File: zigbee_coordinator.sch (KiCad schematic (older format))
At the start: 51 parts, among them J1 USB_C_Receptacle_USB2.0, J2 SWD_POGO_PADS, J3 UART_POGO_PADS, J4 SWD_POGO, J5 SWD_CASTELLATED, J6 UART_CASTELLATED, J7 UART_POGO, Q1 Q_PMOS_GSD, Q2 2N7002, U1 93LCxxBxxOT, U2 MCP1603-OS, U3 FT232H, U4 74LVC126, Y1 12MHz

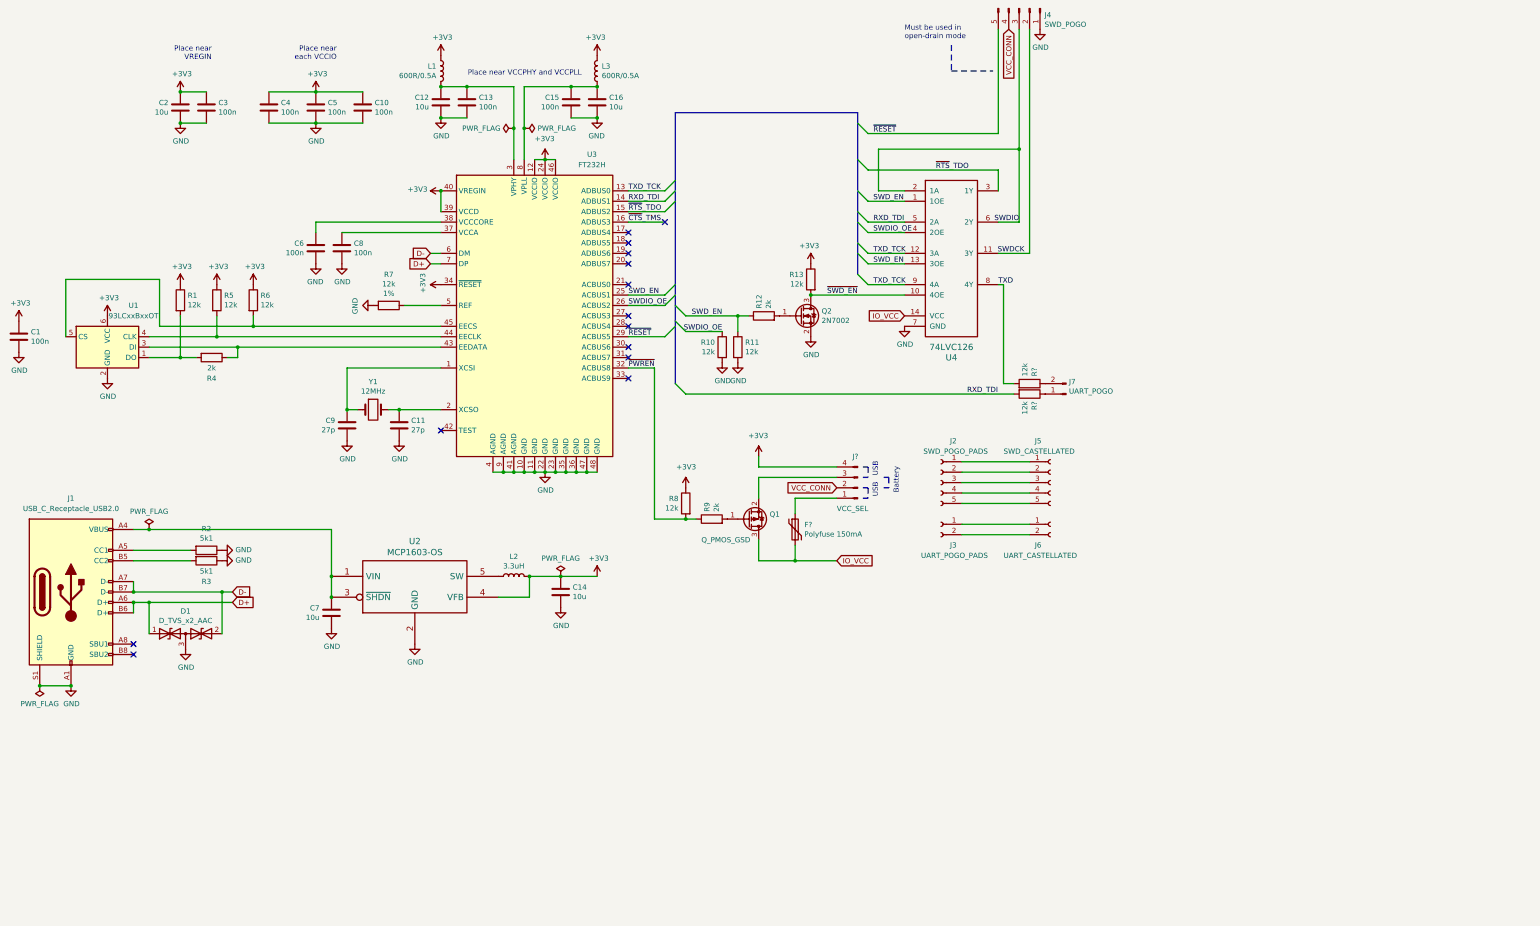
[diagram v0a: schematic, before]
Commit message: First alpha release
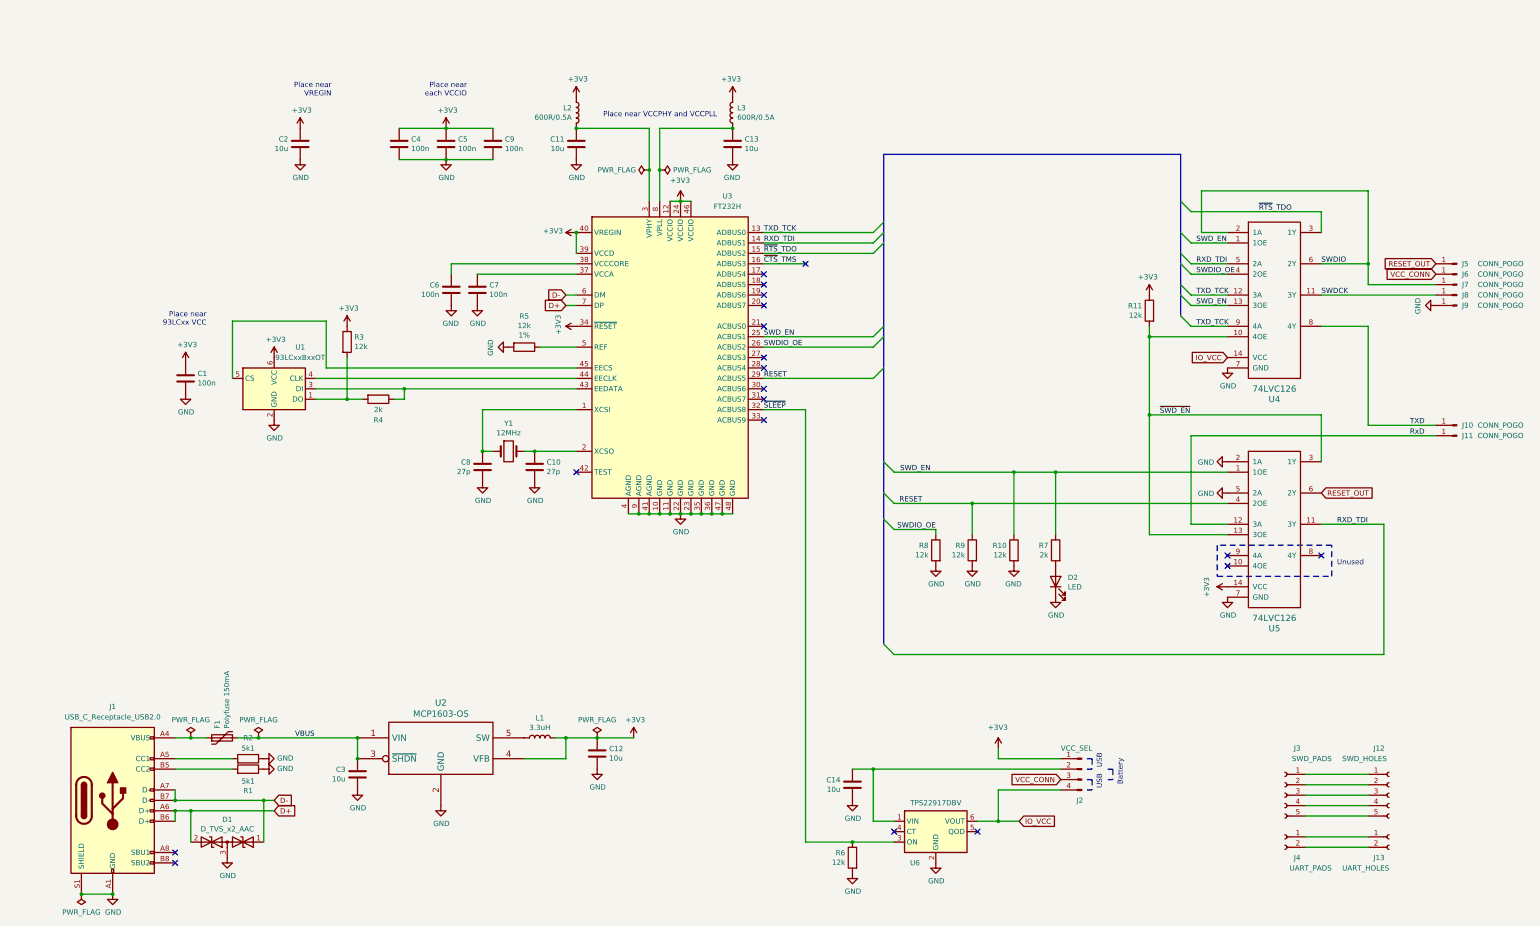
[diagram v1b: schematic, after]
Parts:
- removed C13, C15, C3: 100n, Capacitor_SMD:C_0805_2012Metric, symbol Device:C
- removed J2: SWD_POGO_PADS, symbol Connector:Conn_01x05_Female
- removed J3: UART_POGO_PADS, symbol Connector:Conn_01x02_Female
- removed J4: SWD_POGO, symbol Connector:Conn_01x05_Male
- removed J7: UART_POGO, symbol Connector:Conn_01x02_Male
- removed Q1: Q_PMOS_GSD, Inductor_SMD:L_0805_2012Metric, symbol Device:Q_PMOS_GSD
- removed Q2: 2N7002, Package_TO_SOT_SMD:SOT-23, symbol Transistor_FET:2N7002
- removed R12, R9: 2k, Resistor_SMD:R_0805_2012Metric, symbol Device:R
- removed R5, R6, R? (x2): 12k, Resistor_SMD:R_0805_2012Metric, symbol Device:R
- added C14: 10u, Capacitor_SMD:C_0805_2012Metric, symbol Device:C
- added D2: LED, LED_SMD:LED_0805_2012Metric, symbol Device:LED
- added J10, J11, J5, J6, J7, J8, J9: CONN_POGO, pogopin:pogopin, symbol Connector:Conn_01x01_Male
- added J3: SWD_PADS, pogopin:SWD_pads, symbol Connector:Conn_01x05_Female
- added J4: UART_PADS, pogopin:UART_pads, symbol Connector:Conn_01x02_Female
- added R10: 12k, Resistor_SMD:R_0805_2012Metric, symbol Device:R
- added R7: 2k, Resistor_SMD:R_0805_2012Metric, symbol Device:R
- added U5: 74LVC126, Package_SO:TSSOP-14_4.4x5mm_P0.65mm, symbol 74hc126:74HC126
- added U6: TPS22917DBV, Package_TO_SOT_SMD:SOT-23-6, symbol Power_Management:TPS22917DBV
- F1: renamed from F?; footprint (none) -> Fuse:Fuse_0805_2012Metric
- J12: renamed from J5; value SWD_CASTELLATED -> SWD_HOLES; footprint (none) -> pogopin:SWD_holes
- J13: renamed from J6; value UART_CASTELLATED -> UART_HOLES; footprint (none) -> pogopin:UART_holes
- J2: renamed from J?; footprint (none) -> Connector_PinHeader_1.27mm:PinHeader_1x04_P1.27mm_Horizontal
- Y1: footprint Crystal:Crystal_SMD_HC49-SD -> Crystal:Crystal_SMD_0603-2Pin_6.0x3.5mm
- renumbered C11 to C10, C12 to C11, C14 to C12, C16 to C13, C7 to C3, C8 to C7, C9 to C8, C10 to C9, L2 to L1, L1 to L2, R2 to R1, R13 to R11, R3 to R2, R1 to R3, R7 to R5, R8 to R6, R10 to R8, R11 to R9
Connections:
- net +3V3: now also J2.1 (Pin_1), U5.14 (VCC); no longer J2.4 (Pin_4), R6.1
- net D+: now also D1.2 (A2); no longer D1.1 (A1)
- net D-: now also D1.1 (A1); no longer D1.2 (A2)
- net GND: now also R6.2, C14.2, D2.1 (K), J9.1 (Pin_1), R10.2, U5.2 (1A), U5.5 (2A), U5.7 (GND), U6.2 (GND)
- net IO_VCC: now also J2.4 (Pin_4), U6.6 (VOUT); no longer F1.2
- net RXD_TDI: now also U5.11 (3Y)
- net SWDCK: now also J8.1 (Pin_1)
- net SWDIO: now also J7.1 (Pin_1)
- net SWD_EN: now also R10.1, R7.1, U5.1 (1OE); no longer R9.1
- net TXD: now also J10.1 (Pin_1)
- net VCC_CONN: now also J2.3 (Pin_3), J6.1 (Pin_1); no longer J2.2 (Pin_2)
- net ~SWD_EN: now also U5.13 (3OE), U5.3 (1Y)
- net at J1.A4 (VBUS), J1.A9 (VBUS), J1.B4 (VBUS)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: now also F1.1; no longer C3.1, U2.1 (VIN), U2.3 (~SHDN~)
- net at J1.A5 (CC1): now also R2.2; no longer R1.2
- net at J1.B5 (CC2): now also R1.2; no longer R2.2
- net at J12.1 (Pin_1): now also J3.1 (Pin_1)
- net at J12.2 (Pin_2): now also J3.2 (Pin_2)
- net at J12.3 (Pin_3): now also J3.3 (Pin_3)
- net at J12.4 (Pin_4): now also J3.4 (Pin_4)
- net at J12.5 (Pin_5): now also J3.5 (Pin_5)
- net at J13.1 (Pin_1): now also J4.1 (Pin_1)
- net at J13.2 (Pin_2): now also J4.2 (Pin_2)
- net ~PWREN renamed ~SLEEP
- net ~SLEEP: now also R6.1, U6.3 (ON); no longer R6.2
- net ~RESET renamed RESET
- net RESET: now also R9.1, U5.4 (2OE)
- new net: C14.1, J2.2 (Pin_2), U6.1 (VIN)
- new net: D2.2 (A), R7.2
- new net RESET_OUT: J5.1 (Pin_1), U5.6 (2Y)
- new net RxD: J11.1 (Pin_1), U5.12 (3A)
- new net VBUS: C3.1, F1.2, U2.1 (VIN), U2.3 (~SHDN~)
- no-connect marks 14 -> 19
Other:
- note added: "Place near\n93LCxx VCC"
- note added: "Unused"
- note removed: "Must be used in\nopen-drain mode"
- moved on the sheet: C1, C10, C11, C12, C13, C2, C3, C4, C5, C6, C7, C8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
